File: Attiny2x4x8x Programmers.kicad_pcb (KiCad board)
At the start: 2 copper layers, 33 x 66 mm, 12 parts, among them J1 Conn_01x15_Pin, J2 Conn_01x15_Pin, J3 ICSP, U1 ATtiny84-20P, U2 ATtiny85V-10P

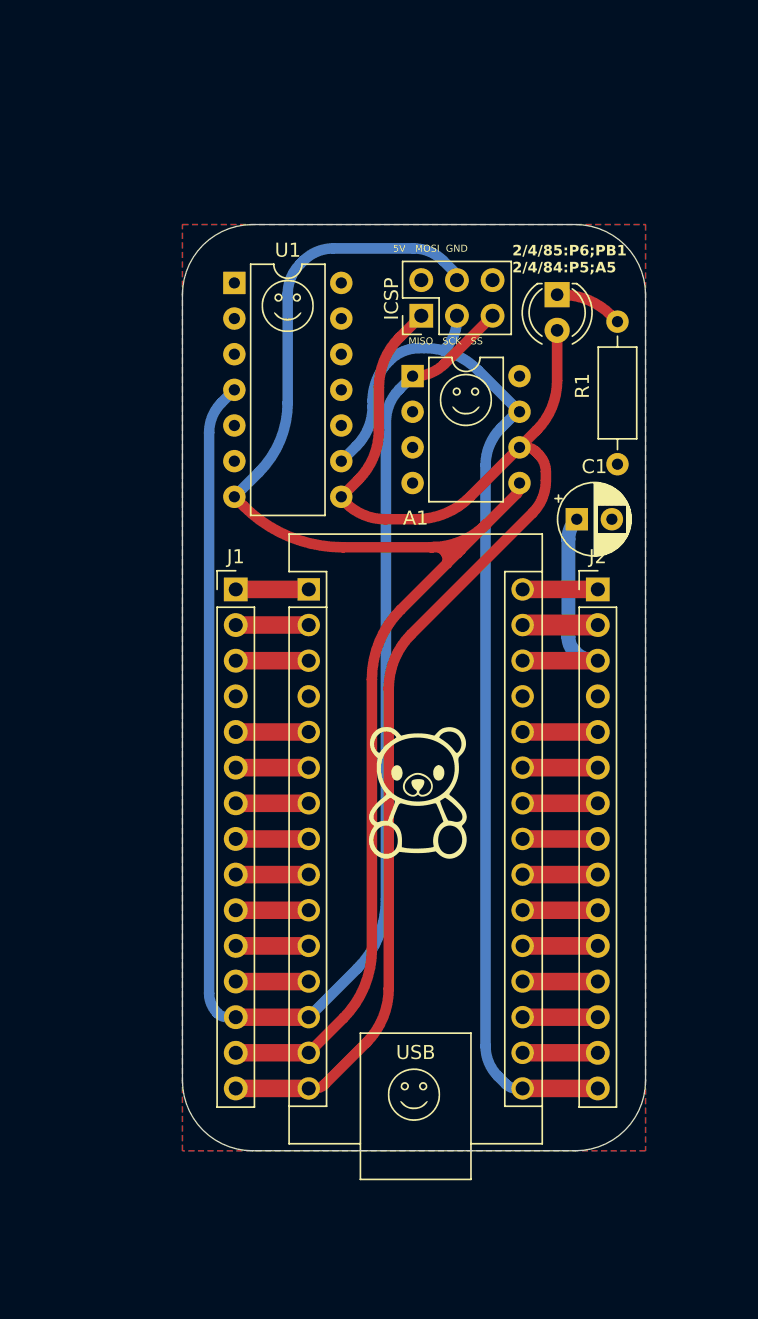
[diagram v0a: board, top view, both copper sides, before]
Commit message: V2
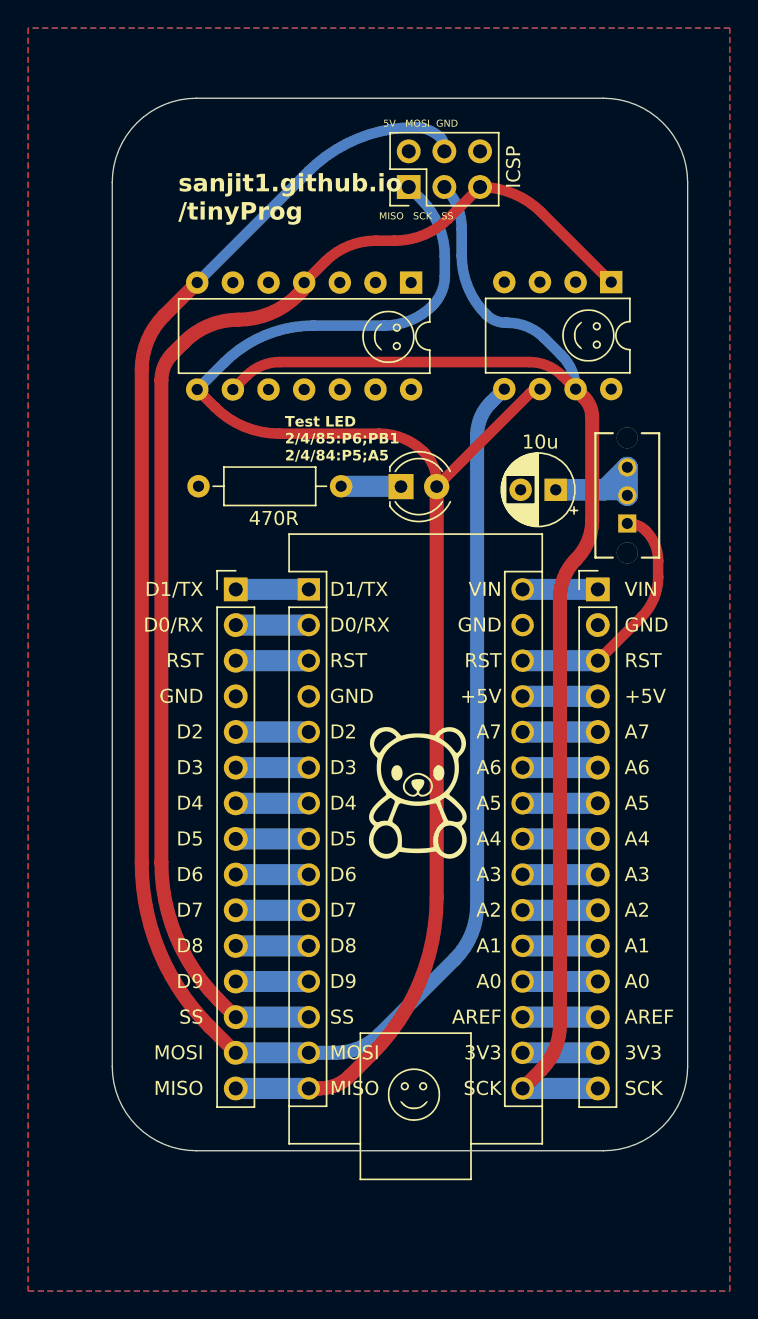
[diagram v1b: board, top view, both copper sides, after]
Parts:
- added G***: LOGO, footprints:GithubQR_14, B.Cu at (87.7, 71.5)
- added SW1: OS102011MS2QN1, OS102011MS2QN1:SPDT_OS102011_CNK, F.Cu at (102.7, 65.3)
- moved R1 22.9 mm to (82.3, 62.6), turned to 180 degrees
- moved D1 17.6 mm to (86.6, 62.7), turned to 0 degrees
- moved U2 15.7 mm to (101.6, 48.1), turned to -90 degrees
- moved U1 12.6 mm to (87.3, 48.1), turned to -90 degrees
- moved G2 9.87 mm to (99.9, 51.9), turned to -90 degrees
- moved J3 9.22 mm to (87.1, 41.3)
- moved G1 7.51 mm to (85.7, 52.0), turned to -90 degrees
- moved C1 2.58 mm to (97.6, 62.9), turned to 180 degrees
- renumbered G*** to G1, G*** to G2, G*** to G3
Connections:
- C1 pad 1: /RST -> Net-(C1-Pad1)
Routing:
- net /MOSI: track 104.3 -> 140.7 mm
- net /SCK: track 77.9 -> 101.5 mm
- net /SS: track 107.3 -> 92.0 mm
- net Net-(C1-Pad1): track 0.00 -> 13.0 mm
- net /MISO: track 97.9 -> 110.7 mm
- net GND: track 5.36 -> 0.00 mm
- net +5V: track 0.00 -> 5.36 mm
- net /RST: track 22.1 -> 23.1 mm
- net Net-(D1-K): track 4.85 -> 4.28 mm
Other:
- board size 33 x 66 mm -> 41 x 75 mm
- board text added: "+5V"
- board text added: "3V3"
- board text added: "A0"
- board text added: "A1"
- board text added: "A2"
- board text added: "A3"
- board text added: "A4"
- board text added: "A5"
- board text added: "A6"
- board text added: "A7"
- board text added: "AREF"
- board text added: "ATTiny Prog"
- board text added: "D0/RX"
- board text added: "D1/TX"
- board text added: "D2"
- board text added: "D3"
- board text added: "D4"
- board text added: "D5"
- board text added: "D6"
- board text added: "D7"
- board text added: "D8"
- board text added: "D9"
- board text added: "GND"
- board text added: "MISO"
- board text added: "MOSI"
- board text added: "RST"
- board text added: "SCK"
- board text added: "SS"
- board text added: "Test LED 2/4/85:P6;PB1 2/4/84:P5;A5"
- board text added: "VIN"
- board text added: "sanjit1.github.io /tinyProg"
- board text removed: "2/4/85:P6;PB1 2/4/84:P5;A5"
